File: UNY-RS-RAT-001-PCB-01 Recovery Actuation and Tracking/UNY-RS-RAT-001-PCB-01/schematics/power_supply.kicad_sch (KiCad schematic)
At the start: 0 parts

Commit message: First draft for ERBUS, Power & CPU
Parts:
- added C1: 10µ, symbol Device:C
- added Q1: STD95P3LLH6AG, Package_TO_SOT_SMD:TO-252-2, symbol Simulation_SPICE:PMOS
- added Q2: NTR4003NT1G, PCM_4ms_Package_SOT:SOT-23, symbol Simulation_SPICE:NMOS
- added R1, R6: 1k, symbol Device:R
- added R2: 560, symbol Device:R
- added R3, R4: 10k, symbol Device:R
- added R5: 3k16, symbol Device:R
- added U1: LGA-16EP_171011801, MagIC_SMD_Wurth:U_Wurth_WPME-VDLM-LGA-16EP, symbol MagIC_Wurth_WPME-VDLM:LGA-16EP_171011801
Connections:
- new net: Q2.1 (G), R2.2
- new net: Q1.1 (G), Q2.3 (D), R1.2
- new net: R4.2, R5.1, U1.13 (FB)
- new net: R6.2, U1.16 (EN)
- new net: U1.14 (NC), U1.15 (NC), U1.5 (NC), U1.6 (NC), U1.7 (NC), U1.8 (NC)
- new net +12V: Q1.2 (D), U1.1 (VIN), U1.2 (VIN), U1.3 (VIN), U1.4 (VIN)
- new net +3V3: C1.1, R4.1, U1.10 (VOUT), U1.11 (VOUT), U1.12 (VOUT), U1.9 (VOUT)
- new net 12V_IN_RAW: Q1.3 (S), R1.1
- new net 5V_PFC: R2.1, R3.2, R6.1
- new net GND: C1.2, Q2.2 (S), R3.1, R5.2, U1.EP (PGND)
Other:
- note added: "3V3 converter"
- note added: "On/Off switch via 5V supply"
- note added: "VGS < -2,5V: an G = 0V AN G = ~ 10V: aus"
- title: RAT High level schematics -> Sensor MCU

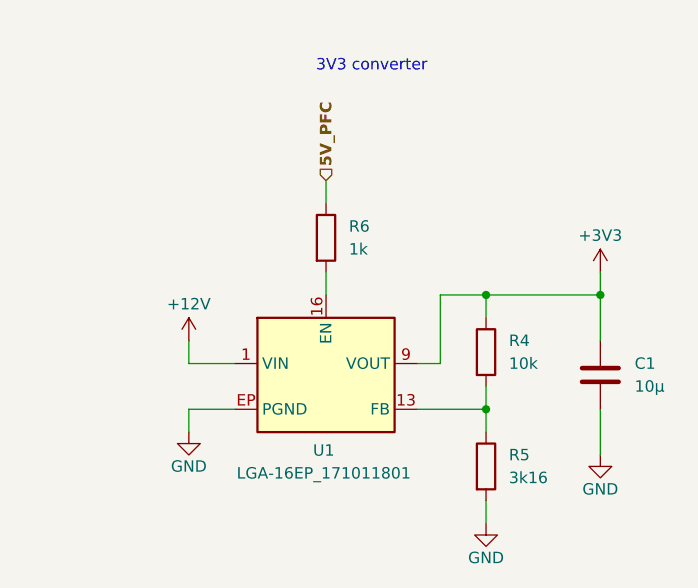
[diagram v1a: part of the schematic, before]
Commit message: Semi complete, missing footprints and connectors
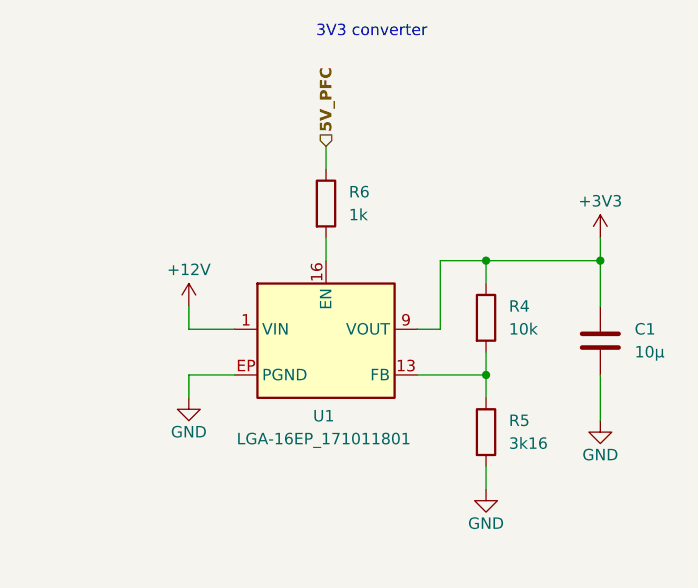
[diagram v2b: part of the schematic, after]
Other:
- company: (none) -> E.R.I.G. e.V
- title: Sensor MCU -> Power Conversion
- moved on the sheet: C1, R4, R5, R6, U1
